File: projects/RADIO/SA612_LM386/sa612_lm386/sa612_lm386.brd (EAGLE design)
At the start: 75 x 50 mm, 43 parts, among them IC1 SA612AN_01,112, IC2 LM386M-1, IC3 LM1117MPX-33NOPB, Q1 BF245

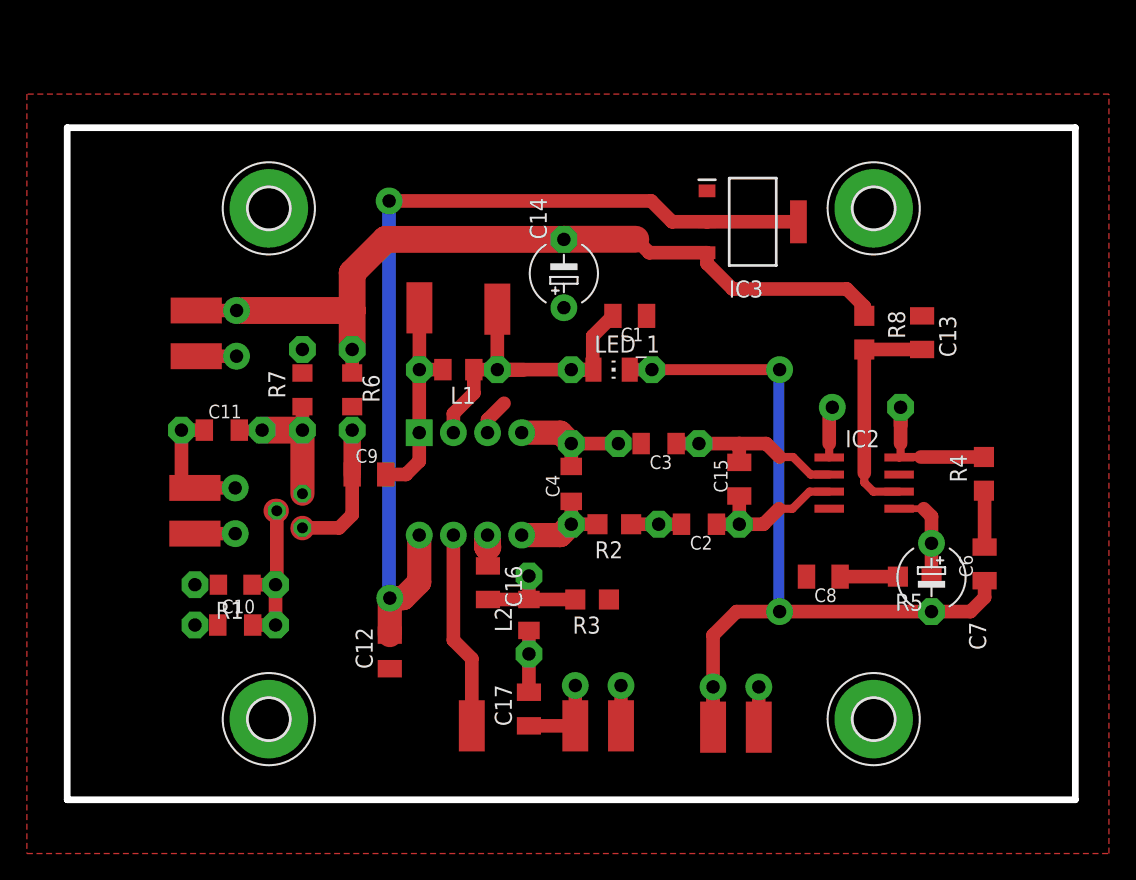
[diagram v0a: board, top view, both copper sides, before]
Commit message: Update
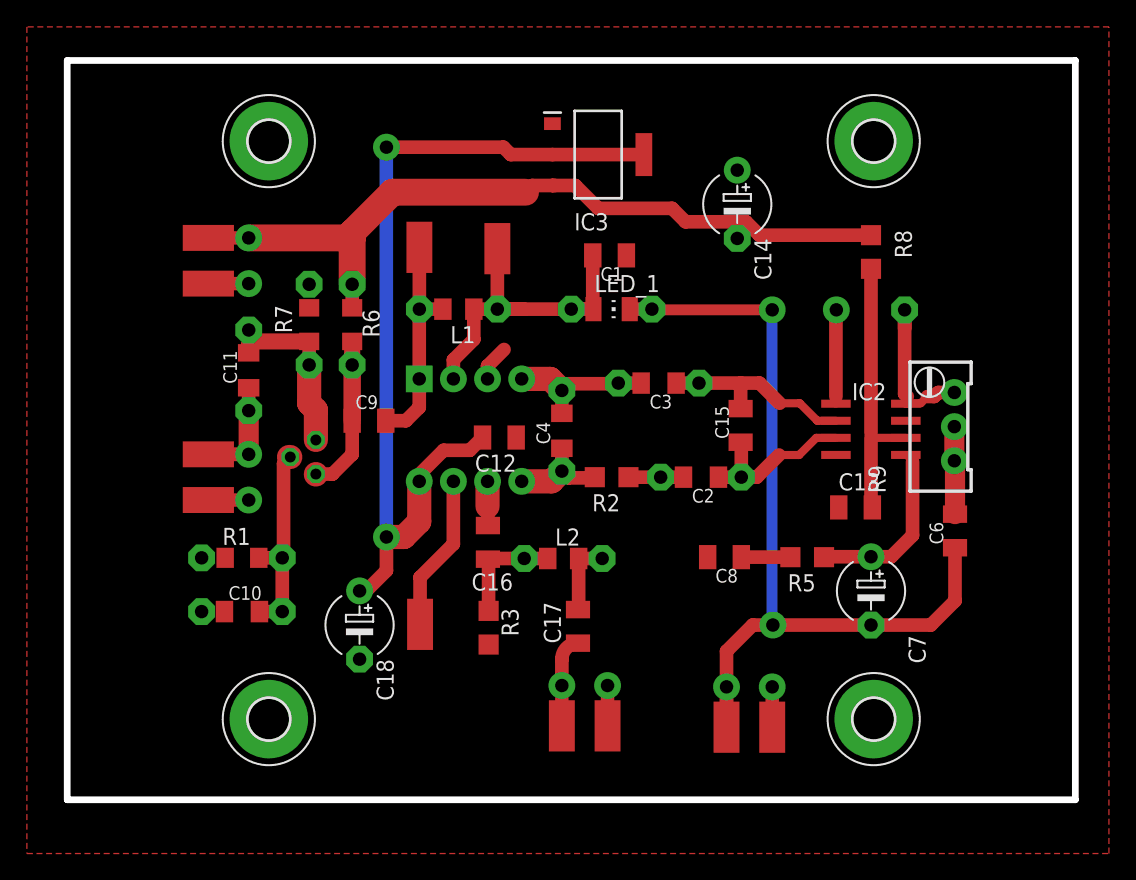
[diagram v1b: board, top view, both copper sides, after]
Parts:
- removed R4: 10k, mylib:R0805W
- added C18: 10uF, mylib:E5-5
- added R9: (no value), rcl:RTRIM64W
- moved C12 17.9 mm to (32.1, 26.9), turned to 180 degrees
- moved C13 13.9 mm to (58.6, 21.8), turned to 0 degrees
- moved C14 13.9 mm to (49.9, 44.3), turned to 270 degrees
- moved IC3 12.5 mm to (39.5, 48.0)
- moved P_1 8.47 mm to (26.2, 13.1)
- moved R5 8.13 mm to (55.1, 18.1)
- moved R3 7.98 mm to (31.4, 12.8), turned to 90 degrees
- moved C8 7.49 mm to (48.9, 18.1)
- moved C5 7.26 mm to (59.8, 36.5)
- moved C17 7.15 mm to (38.0, 12.9)
- moved R8 6.02 mm to (59.8, 40.8)
- moved CON_2 5.47 mm to (10.5, 40.1)
- moved H3 5.00 mm to (15.0, 49.0)
- moved H4 5.00 mm to (60.0, 49.0)
- moved L2 4.91 mm to (36.9, 17.9), turned to 180 degrees
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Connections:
- net 5V: now also C18.+
- net GND: now also C18.-
- net N$12: now also R9.3; no longer R4.2
- net N$13: now also R9.1, R9.2; no longer R4.1
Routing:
- net N$15: track 7.13 -> 13.7 mm
- net 5V: track 69.6 -> 65.8 mm
- net N$14: track 58.7 -> 62.3 mm
- net N$21: track 17.1 -> 20.4 mm
- net N$19: track 11.2 -> 14.4 mm
- net N$11: track 3.84 -> 7.01 mm
- net N$17: track 12.1 -> 15.3 mm
- net N$10: track 14.8 -> 11.7 mm
- net N$13: track 4.22 -> 6.53 mm
- net 12V: track 58.4 -> 56.4 mm
- net N$8: track 9.23 -> 11.2 mm
- net N$18: track 10.4 -> 11.7 mm
- net N$4: track 13.7 -> 15.0 mm
- net N$3: track 11.5 -> 12.6 mm
- net N$9: track 2.30 -> 3.30 mm
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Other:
- board size 75 x 50 mm -> 75 x 55 mm
